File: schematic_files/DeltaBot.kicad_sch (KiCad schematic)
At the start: 16 parts, among them J1 USB C PD Modulle, J2 LIDAR, J3 MOTOR_L, J4 MOTOR_R, SW1 SW_SPDT, U1 Radxa_ROCK5B, U2 Buck Converter

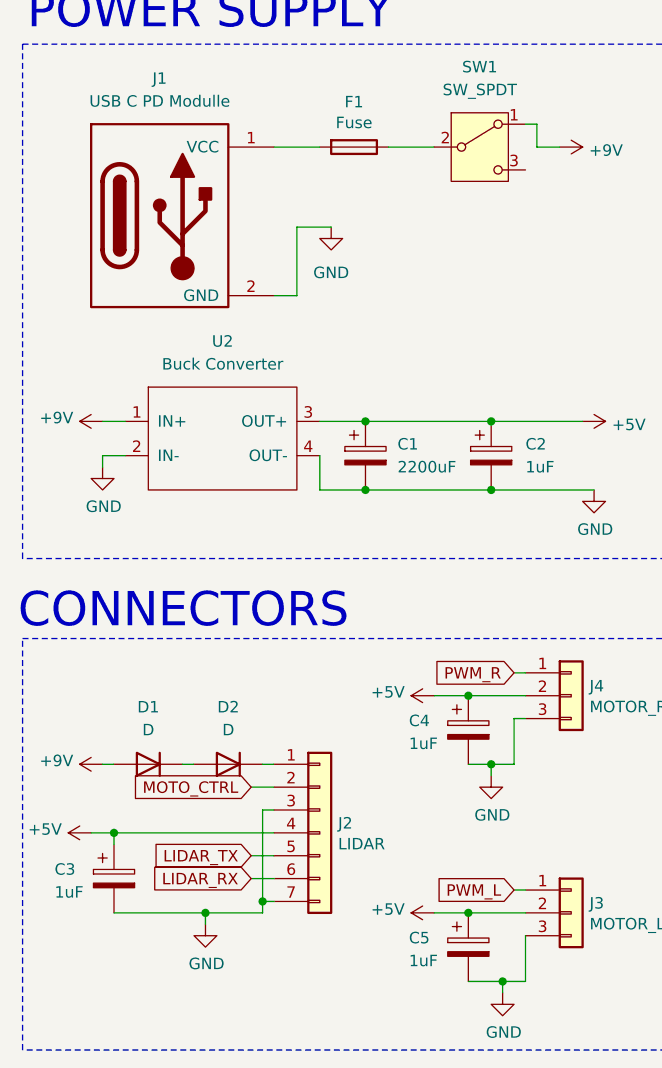
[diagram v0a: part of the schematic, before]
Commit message: Updated PCB layout
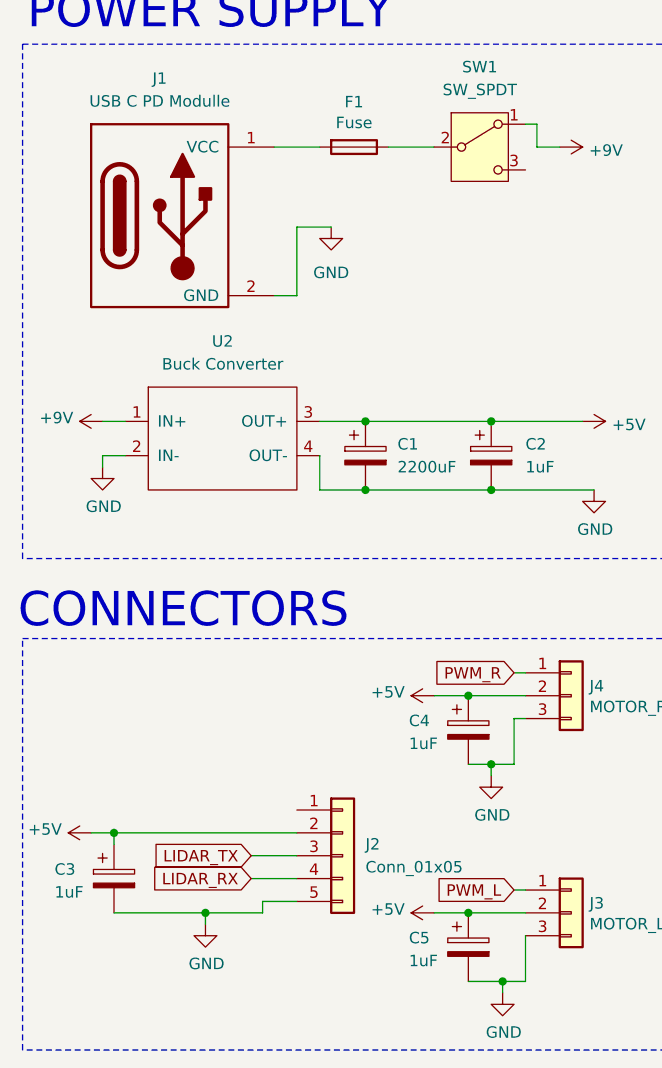
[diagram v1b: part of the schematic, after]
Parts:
- removed D1, D2: D, deltabot:D_DO-41_SOD81_P10.16mm_Horizontal, symbol Device:D
- removed J2: LIDAR, deltabot:PinHeader_1x07_P2.54mm_Vertical, symbol Connector_Generic:Conn_01x07
- added J2: Conn_01x05, Connector_PinHeader_2.54mm:PinHeader_1x05_P2.54mm_Vertical, symbol Connector_Generic:Conn_01x05
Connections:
- net +5V: now also J2.2 (Pin_2)
- net GND: now also J2.5 (Pin_5)
- net LIDAR_RX: now also J2.4 (Pin_4)
- net LIDAR_TX: now also J2.3 (Pin_3)

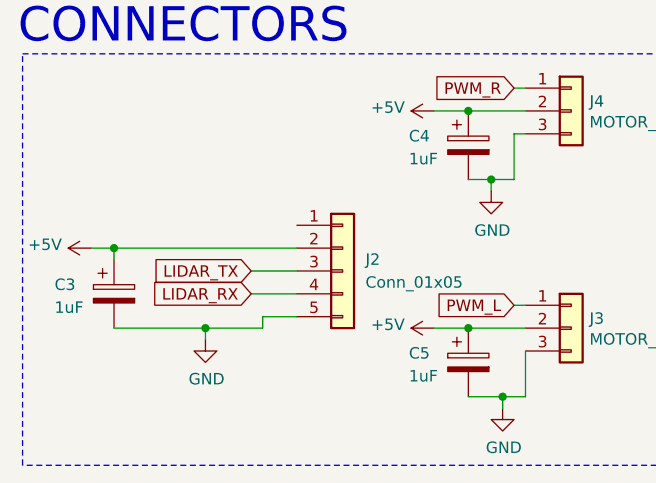
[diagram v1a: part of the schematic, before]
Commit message: Small changes
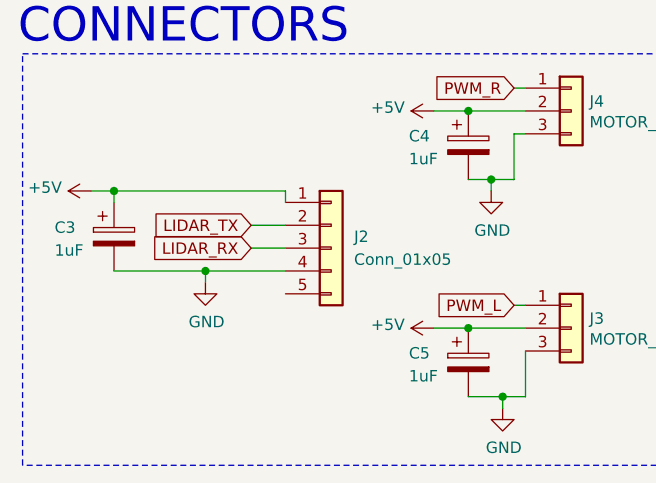
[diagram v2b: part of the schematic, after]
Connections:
- net +5V: now also J2.1 (Pin_1); no longer J2.2 (Pin_2)
- net GND: now also J2.4 (Pin_4); no longer J2.5 (Pin_5)
- net LIDAR_RX: now also J2.3 (Pin_3); no longer J2.4 (Pin_4)
- net LIDAR_TX: now also J2.2 (Pin_2); no longer J2.3 (Pin_3)
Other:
- moved on the sheet: C3, J2
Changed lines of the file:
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@@
 	)
 	(junction
-		(at 34.29 119.38)
+		(at 24.13 104.14)
 		(diameter 0)
 		(color 0 0 0 0)
@@
 	)
 	(junction
-		(at 24.13 110.49)
+		(at 34.29 113.03)
 		(diameter 0)
 		(color 0 0 0 0)
@@
 	(wire
 		(pts
-			(xy 22.86 68.58) (xy 22.86 69.85)
+			(xy 34.29 113.03) (xy 34.29 114.3)
 		)
 		(stroke
@@
 	(wire
 		(pts
-			(xy 24.13 119.38) (xy 34.29 119.38)
+			(xy 22.86 68.58) (xy 22.86 69.85)
 		)
 		(stroke
@@
 	(wire
 		(pts
-			(xy 101.6 76.2) (xy 106.68 76.2)
+			(xy 24.13 113.03) (xy 34.29 113.03)
 		)
 		(stroke
@@
 	(wire
 		(pts
-			(xy 24.13 110.49) (xy 44.45 110.49)
+			(xy 101.6 76.2) (xy 106.68 76.2)
 		)
 		(stroke
@@
 	(wire
 		(pts
+			(xy 39.37 107.95) (xy 43.18 107.95)
+		)
+		(stroke
+			(width 0)
+			(type default)
+		)
+	)
+	(wire
+		(pts
 			(xy 66.04 64.77) (xy 76.2 64.77)
 		)
@@
 	(wire
 		(pts
-			(xy 34.29 119.38) (xy 40.64 119.38)
+			(xy 66.04 72.39) (xy 77.47 72.39)
 		)
 		(stroke
@@
 	(wire
 		(pts
-			(xy 66.04 72.39) (xy 77.47 72.39)
+			(xy 43.18 113.03) (xy 34.29 113.03)
 		)
 		(stroke
@@
 	(wire
 		(pts
-			(xy 68.58 97.79) (xy 68.58 102.87)
+			(xy 24.13 104.14) (xy 43.18 104.14)
 		)
 		(stroke
@@
 	(wire
 		(pts
-			(xy 104.14 83.82) (xy 106.68 83.82)
+			(xy 68.58 97.79) (xy 68.58 102.87)
 		)
 		(stroke
@@
 	(wire
 		(pts
-			(xy 66.04 102.87) (xy 68.58 102.87)
+			(xy 104.14 83.82) (xy 106.68 83.82)
 		)
 		(stroke
@@
 	(wire
 		(pts
-			(xy 40.64 119.38) (xy 40.64 118.11)
+			(xy 66.04 102.87) (xy 68.58 102.87)
 		)
 		(stroke
@@
 	(wire
 		(pts
-			(xy 24.13 111.76) (xy 24.13 110.49)
+			(xy 24.13 105.41) (xy 24.13 104.14)
 		)
 		(stroke
@@
 	(wire
 		(pts
-			(xy 34.29 120.65) (xy 34.29 119.38)
-		)
-		(stroke
-			(width 0)
-			(type default)
-		)
-	)
-	(wire
-		(pts
 			(xy 46.99 72.39) (xy 46.99 68.58)
 		)
@@
 	(wire
 		(pts
-			(xy 39.37 113.03) (xy 44.45 113.03)
-		)
-		(stroke
-			(width 0)
-			(type default)
-		)
-	)
-	(wire
-		(pts
 			(xy 22.86 64.77) (xy 25.4 64.77)
 		)
@@
 	(wire
 		(pts
+			(xy 39.37 110.49) (xy 43.18 110.49)
+		)
+		(stroke
+			(width 0)
+			(type default)
+		)
+	)
+	(wire
+		(pts
 			(xy 71.12 34.29) (xy 73.66 34.29)
 		)
@@
 	(wire
 		(pts
-			(xy 39.37 115.57) (xy 44.45 115.57)
-		)
-		(stroke
-			(width 0)
-			(type default)
-		)
-	)
-	(wire
-		(pts
 			(xy 168.91 26.67) (xy 176.53 26.67)
 		)
@@
 	(wire
 		(pts
-			(xy 40.64 118.11) (xy 44.45 118.11)
+			(xy 168.91 35.56) (xy 167.64 35.56)
 		)
 		(stroke
@@
 	(wire
 		(pts
-			(xy 168.91 35.56) (xy 167.64 35.56)
+			(xy 71.12 31.75) (xy 71.12 34.29)
 		)
 		(stroke
@@
 	(wire
 		(pts
-			(xy 71.12 31.75) (xy 71.12 34.29)
+			(xy 43.18 105.41) (xy 43.18 104.14)
 		)
 		(stroke
@@
 	(wire
 		(pts
-			(xy 21.59 110.49) (xy 24.13 110.49)
+			(xy 21.59 104.14) (xy 24.13 104.14)
 		)
 		(stroke
@@
 	(global_label "LIDAR_TX"
 		(shape input)
-		(at 39.37 113.03 180)
+		(at 39.37 107.95 180)
 		(effects
 			(font
@@
 		)
 		(property "Intersheetrefs" "${INTERSHEET_REFS}"
-			(at 39.37 113.03 0)
+			(at 39.37 107.95 0)
 			(effects
 				(font
@@
 	(global_label "LIDAR_RX"
 		(shape input)
-		(at 39.37 115.57 180)
+		(at 39.37 110.49 180)
 		(effects
 			(font
@@
 		)
 		(property "Intersheetrefs" "${INTERSHEET_REFS}"
-			(at 39.37 115.57 0)
+			(at 39.37 110.49 0)
 			(effects
 				(font
@@
 	(symbol
 		(lib_id "power:GND")
-		(at 34.29 120.65 0)
+		(at 34.29 114.3 0)
 		(unit 1)
 		(exclude_from_sim no)
@@
 		(dnp no)
 		(property "Reference" "#PWR09"
-			(at 34.29 127 0)
+			(at 34.29 120.65 0)
 			(effects
 				(font
@@
 		)
 		(property "Value" "GND"
-			(at 34.417 125.0442 0)
+			(at 34.417 118.6942 0)
 			(effects
 				(font
@@
 		)
 		(property "Footprint" ""
-			(at 34.29 120.65 0)
+			(at 34.29 114.3 0)
 			(effects
 				(font
@@
 		)
 		(property "Datasheet" ""
-			(at 34.29 120.65 0)
+			(at 34.29 114.3 0)
 			(effects
 				(font
@@
 		)
 		(property "Description" ""
-			(at 34.29 120.65 0)
+			(at 34.29 114.3 0)
 			(effects
 				(font
@@
 	(symbol
 		(lib_id "power:+5V")
-		(at 21.59 110.49 90)
+		(at 21.59 104.14 90)
 		(unit 1)
 		(exclude_from_sim no)
@@
 		(dnp no)
 		(property "Reference" "#PWR08"
-			(at 25.4 110.49 0)
+			(at 25.4 104.14 0)
 			(effects
 				(font
@@
 		)
 		(property "Value" "+5V"
-			(at 18.3388 110.109 90)
+			(at 18.3388 103.759 90)
 			(effects
 				(font
@@
 		)
 		(property "Footprint" ""
-			(at 21.59 110.49 0)
+			(at 21.59 104.14 0)
 			(effects
 				(font
@@
 		)
 		(property "Datasheet" ""
-			(at 21.59 110.49 0)
+			(at 21.59 104.14 0)
 			(effects
 				(font
@@
 		)
 		(property "Description" ""
-			(at 21.59 110.49 0)
+			(at 21.59 104.14 0)
 			(effects
 				(font
@@
 	(symbol
 		(lib_id "Connector_Generic:Conn_01x05")
-		(at 49.53 113.03 0)
+		(at 48.26 110.49 0)
 		(unit 1)
 		(exclude_from_sim no)
@@
 		(fields_autoplaced yes)
 		(property "Reference" "J2"
-			(at 52.07 111.7599 0)
+			(at 50.8 109.2199 0)
 			(effects
 				(font
@@
 		)
 		(property "Value" "Conn_01x05"
-			(at 52.07 114.2999 0)
+			(at 50.8 111.7599 0)
 			(effects
 				(font
@@
 		)
 		(property "Footprint" "Connector_PinHeader_2.54mm:PinHeader_1x05_P2.54mm_Vertical"
-			(at 49.53 113.03 0)
+			(at 48.26 110.49 0)
 			(effects
 				(font
@@
 		)
 		(property "Datasheet" "~"
-			(at 49.53 113.03 0)
+			(at 48.26 110.49 0)
 			(effects
 				(font
@@
 		)
 		(property "Description" "Generic connector, single row, 01x05, script generated (kicad-library-utils/schlib/autogen/connector/)"
-			(at 49.53 113.03 0)
+			(at 48.26 110.49 0)
 			(effects
 				(font
@@
 	(symbol
 		(lib_id "Device:C_Polarized")
-		(at 24.13 115.57 0)
+		(at 24.13 109.22 0)
 		(unit 1)
 		(exclude_from_sim no)
@@
 		(dnp no)
 		(property "Reference" "C3"
-			(at 17.526 114.554 0)
+			(at 17.526 108.204 0)
 			(effects
 				(font
@@
 		)
 		(property "Value" "1uF"
-			(at 17.526 117.094 0)
+			(at 17.526 110.744 0)
 			(effects
 				(font
@@
 		)
 		(property "Footprint" "deltabot:C_Disc_D3.0mm_W2.0mm_P2.50mm"
-			(at 25.0952 119.38 0)
+			(at 25.0952 113.03 0)
 			(effects
 				(font
@@
 		)
 		(property "Datasheet" "~"
-			(at 24.13 115.57 0)
+			(at 24.13 109.22 0)
 			(effects
 				(font
@@
 		)
 		(property "Description" "Polarized capacitor"
-			(at 24.13 115.57 0)
+			(at 24.13 109.22 0)
 			(effects
 				(font
